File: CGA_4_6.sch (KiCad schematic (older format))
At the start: 9 parts, among them U1 74S112, U2 74LS74, U26 74S04, U28 74LS10, U29 74S04, U46 74LS00, U47 74LS51, U49 74LS02, U62 74LS125

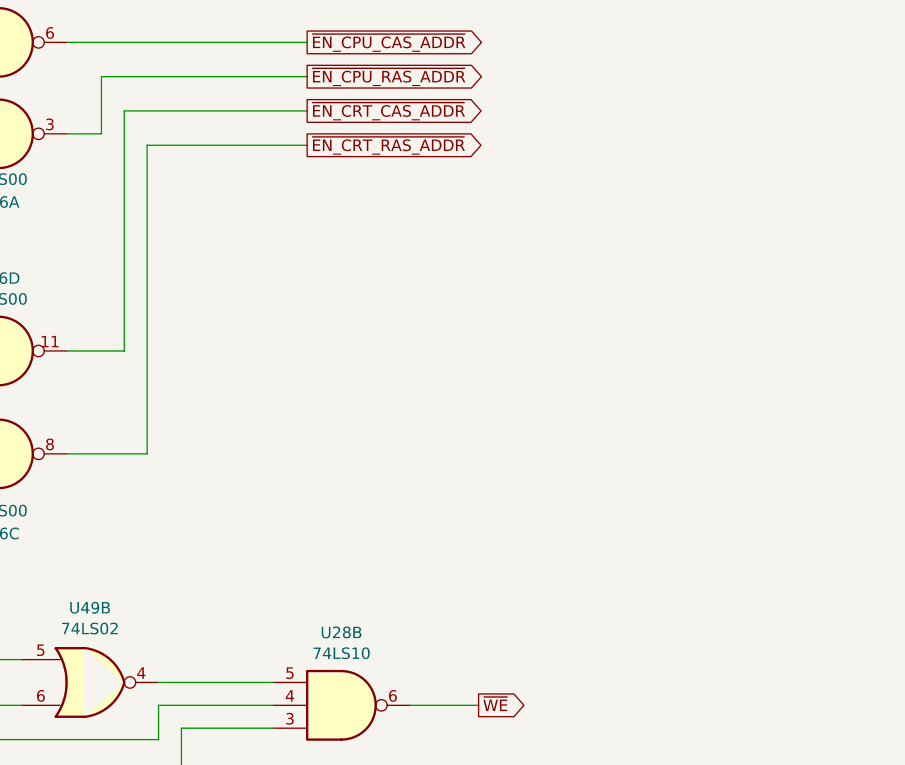
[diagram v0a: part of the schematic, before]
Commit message: More sheet 4
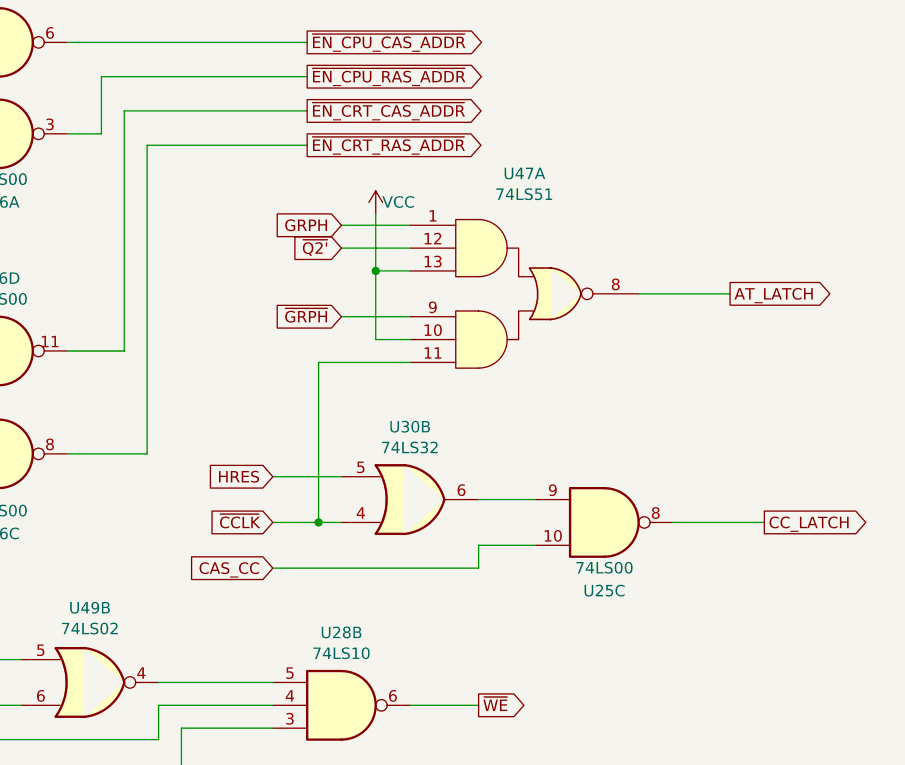
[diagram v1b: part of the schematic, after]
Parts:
- added U25: 74LS00, Package_DIP:DIP-14_W7.62mm_LongPads, symbol 74xx:74LS00
- added U30: 74LS32, Package_DIP:DIP-14_W7.62mm_LongPads, symbol 74xx:74LS32
- added unit 1 of U47
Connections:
- net HRES: now also U30.5
- net VCC: now also U47.10, U47.13
- net ~Q2': now also U47.12
- new net: U25.9, U30.6
- new net AT_LATCH: U47.8
- new net CAS_CC: U25.10
- new net CC_LATCH: U25.8
- new net GRPH: U47.1
- new net ~CCLK: U30.4, U47.11
- new net ~GRPH: U47.9
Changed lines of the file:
@@
 Wire Wire Line
 	4800 5600 4250 5600
+$Comp
+L 74xx:74LS32 U?
+U 2 1 62ED8784
+P 5800 3000
+AR Path="/60463C57/62ED8784" Ref="U?"  Part="3"
+AR Path="/60463CC5/62ED8784" Ref="U30"  Part="2"
+F 0 "U30" H 5800 2683 50  0000 C CNN
+F 1 "74LS32" H 5800 2774 50  0000 C CNN
+F 2 "Package_DIP:DIP-14_W7.62mm_LongPads" H 5800 3000 50  0001 C CNN
+F 3 "http://www.ti.com/lit/gpn/sn74LS32" H 5800 3000 50  0001 C CNN
+	2    5800 3000
+	1    0    0    1
+$EndComp
+Text GLabel 5200 2900 0    50   Input ~ 0
+HRES
+Wire Wire Line
+	5200 2900 5500 2900
+Text GLabel 5200 3100 0    50   Input ~ 0
+~CCLK
+Wire Wire Line
+	5500 3100 5400 3100
+$Comp
+L 74xx:74LS00 U25
+U 3 1 62EFF4A5
+P 6650 3100
+F 0 "U25" H 6650 2800 50  0000 C CNN
+F 1 "74LS00" H 6650 2900 50  0000 C CNN
+F 2 "Package_DIP:DIP-14_W7.62mm_LongPads" H 6650 3100 50  0001 C CNN
+F 3 "http://www.ti.com/lit/gpn/sn74ls00" H 6650 3100 50  0001 C CNN
+	3    6650 3100
+	1    0    0    -1
+$EndComp
+Wire Wire Line
+	6350 3000 6100 3000
+Wire Wire Line
+	6350 3200 6100 3200
+Wire Wire Line
+	6100 3200 6100 3300
+Wire Wire Line
+	6100 3300 5200 3300
+Text GLabel 5200 3300 0    50   Input ~ 0
+CAS_CC
+Wire Wire Line
+	6950 3100 7350 3100
+Text GLabel 7350 3100 2    50   Output ~ 0
+CC_LATCH
+$Comp
+L 74xx:74LS51 U47
+U 1 1 62F37BE3
+P 6300 2100
+F 0 "U47" H 6300 2625 50  0000 C CNN
+F 1 "74LS51" H 6300 2534 50  0000 C CNN
+F 2 "Package_DIP:DIP-14_W7.62mm_LongPads" H 6300 2100 50  0001 C CNN
+F 3 "http://www.ti.com/lit/ds/symlink/sn74ls51.pdf" H 6300 2100 50  0001 C CNN
+	1    6300 2100
+	1    0    0    -1
+$EndComp
+Wire Wire Line
+	6800 2100 7200 2100
+Text GLabel 7200 2100 2    50   Output ~ 0
+AT_LATCH
+$Comp
+L power:VCC #PWR?
+U 1 1 62F71B77
+P 5650 1750
+F 0 "#PWR?" H 5650 1600 50  0001 C CNN
+F 1 "VCC" H 5750 1800 50  0000 C CNN
+F 2 "" H 5650 1750 50  0001 C CNN
+F 3 "" H 5650 1750 50  0001 C CNN
+	1    5650 1750
+	1    0    0    -1
+$EndComp
+Text GLabel 5500 1900 0    50   Input ~ 0
+~Q2'
+Wire Wire Line
+	5500 1900 5800 1900
+Wire Wire Line
+	5800 2300 5650 2300
+Wire Wire Line
+	5650 2300 5650 2000
+Wire Wire Line
+	5650 2000 5800 2000
+Wire Wire Line
+	5650 2000 5650 1750
+Connection ~ 5650 2000
+Wire Wire Line
+	5800 2400 5400 2400
+Wire Wire Line
+	5400 2400 5400 3100
+Connection ~ 5400 3100
+Wire Wire Line
+	5400 3100 5200 3100
+Text GLabel 5500 1800 0    50   Input ~ 0
+GRPH
+Wire Wire Line
+	5500 1800 5800 1800
+Text GLabel 5500 2200 0    50   Input ~ 0
+~GRPH
+Wire Wire Line
+	5500 2200 5800 2200
 $EndSCHEMATC
